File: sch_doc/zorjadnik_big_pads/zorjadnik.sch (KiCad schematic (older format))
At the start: 51 parts, among them J1 OUT1, J10 output GND, J11 power supply GND, J12 spare port, J2 OUT2, J3 Vsb, J4 GND, J5 display module, J6 firmware, J7 cooling fan, J9 power supply Vout, Q1 BCR512, Q2 BCR108, Q3 BCR108, U1 AP1117-33, U2 STM32F030F4Px

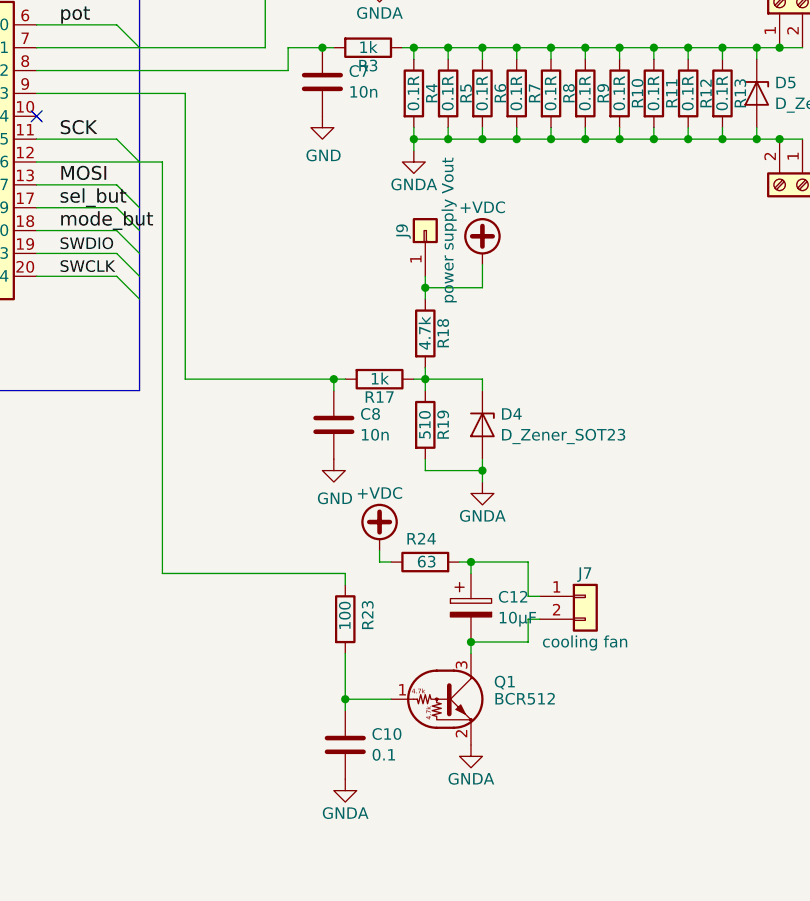
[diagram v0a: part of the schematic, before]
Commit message: что то подкрутил
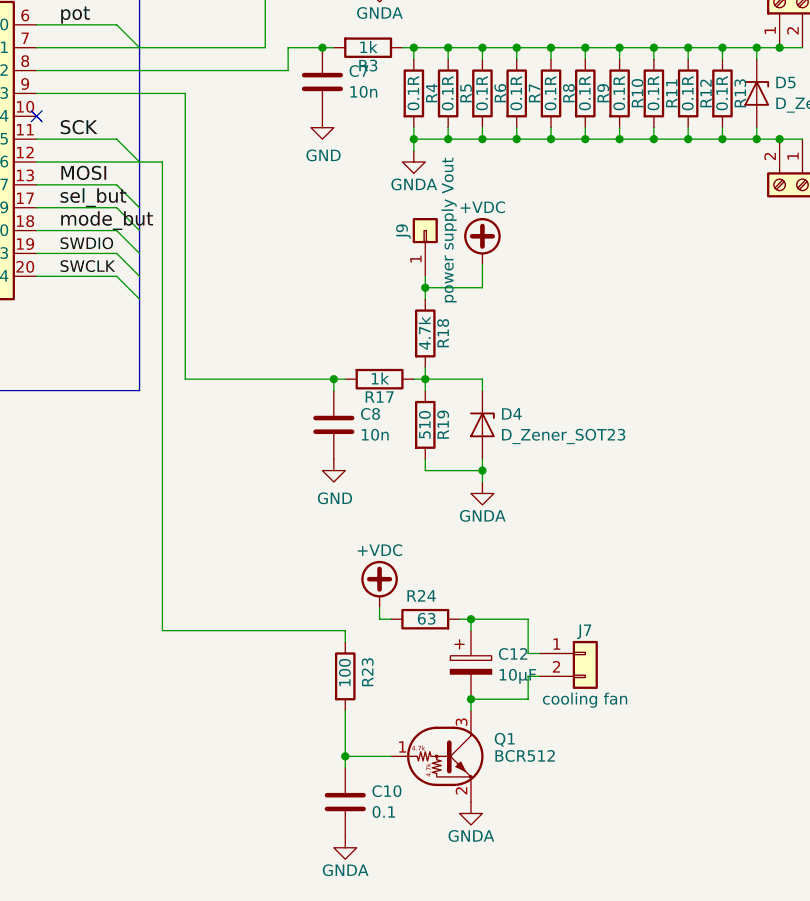
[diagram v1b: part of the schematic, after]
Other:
- moved on the sheet: C10, C12, J7, Q1, R23, R24
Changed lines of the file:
@@
 L led_digits:BCR512 Q1
 U 1 1 5D43E6DF
-P 6100 5900
-F 0 "Q1" H 6300 5975 50  0000 L CNN
-F 1 "BCR512" H 6300 5900 50  0000 L CNN
-F 2 "Package_TO_SOT_SMD:SOT-23" H 6100 5900 50  0001 L CNN
-F 3 "" H 6100 5900 50  0001 L CNN
-	1    6100 5900
+P 6100 6150
+F 0 "Q1" H 6300 6225 50  0000 L CNN
+F 1 "BCR512" H 6300 6150 50  0000 L CNN
+F 2 "Package_TO_SOT_SMD:SOT-23" H 6100 6150 50  0001 L CNN
+F 3 "" H 6100 6150 50  0001 L CNN
+	1    6100 6150
 	1    0    0    -1
 $EndComp
@@
 L zorjadnik-rescue:+VDC-power1 #PWR017
 U 1 1 5D43F586
-P 5800 5250
-F 0 "#PWR017" H 5800 5150 50  0001 C CNN
-F 1 "+VDC" H 5800 5500 50  0000 C CNN
-F 2 "" H 5800 5250 50  0001 C CNN
-F 3 "" H 5800 5250 50  0001 C CNN
-	1    5800 5250
-	1    0    0    -1
-$EndComp
-Wire Wire Line
-	5650 5900 5850 5900
+P 5800 5500
+F 0 "#PWR017" H 5800 5400 50  0001 C CNN
+F 1 "+VDC" H 5800 5750 50  0000 C CNN
+F 2 "" H 5800 5500 50  0001 C CNN
+F 3 "" H 5800 5500 50  0001 C CNN
+	1    5800 5500
+	1    0    0    -1
+$EndComp
+Wire Wire Line
+	5650 6150 5850 6150
 Entry Wire Line
 	4650 3650 4750 3750
@@
 L zorjadnik-rescue:GNDA-power1 #PWR0102
 U 1 1 5D598089
-P 6200 6100
-F 0 "#PWR0102" H 6200 5850 50  0001 C CNN
-F 1 "GNDA" H 6200 5950 50  0000 C CNN
-F 2 "" H 6200 6100 50  0001 C CNN
-F 3 "" H 6200 6100 50  0001 C CNN
-	1    6200 6100
+P 6200 6350
+F 0 "#PWR0102" H 6200 6100 50  0001 C CNN
+F 1 "GNDA" H 6200 6200 50  0000 C CNN
+F 2 "" H 6200 6350 50  0001 C CNN
+F 3 "" H 6200 6350 50  0001 C CNN
+	1    6200 6350
 	1    0    0    -1
 $EndComp
@@
 L zorjadnik-rescue:C-Device1 C10
 U 1 1 5D601FED
-P 5650 6100
-F 0 "C10" H 5765 6146 50  0000 L CNN
-F 1 "0.1" H 5765 6055 50  0000 L CNN
-F 2 "Capacitor_SMD:C_0603_1608Metric" H 5688 5950 50  0001 C CNN
-F 3 "~" H 5650 6100 50  0001 C CNN
-	1    5650 6100
+P 5650 6350
+F 0 "C10" H 5765 6396 50  0000 L CNN
+F 1 "0.1" H 5765 6305 50  0000 L CNN
+F 2 "Capacitor_SMD:C_0603_1608Metric" H 5688 6200 50  0001 C CNN
+F 3 "~" H 5650 6350 50  0001 C CNN
+	1    5650 6350
 	1    0    0    -1
 $EndComp
@@
 L zorjadnik-rescue:GNDA-power1 #PWR0106
 U 1 1 5D602460
-P 5650 6250
-F 0 "#PWR0106" H 5650 6000 50  0001 C CNN
-F 1 "GNDA" H 5650 6100 50  0000 C CNN
-F 2 "" H 5650 6250 50  0001 C CNN
-F 3 "" H 5650 6250 50  0001 C CNN
-	1    5650 6250
-	1    0    0    -1
-$EndComp
-Wire Wire Line
-	5650 5950 5650 5900
-Connection ~ 5650 5900
+P 5650 6500
+F 0 "#PWR0106" H 5650 6250 50  0001 C CNN
+F 1 "GNDA" H 5650 6350 50  0000 C CNN
+F 2 "" H 5650 6500 50  0001 C CNN
+F 3 "" H 5650 6500 50  0001 C CNN
+	1    5650 6500
+	1    0    0    -1
+$EndComp
+Wire Wire Line
+	5650 6200 5650 6150
+Connection ~ 5650 6150
 NoConn ~ 4300 3350
 Entry Wire Line
@@
 	5800 2750 5800 2700
 Wire Wire Line
-	4850 3550 4850 5350
-Wire Wire Line
-	4850 5350 5650 5350
+	4850 5600 5650 5600
 Wire Wire Line
 	5600 4500 4950 4500
@@
 	5300 2600 5450 2600
 Wire Wire Line
-	5650 5350 5650 5400
-Wire Wire Line
-	5650 5900 5650 5700
+	5650 5600 5650 5650
+Wire Wire Line
+	5650 6150 5650 5950
 $Comp
 L zorjadnik-rescue:R-Device1 R23
 U 1 1 5D4C7FD8
-P 5650 5550
-F 0 "R23" V 5750 5500 50  0000 L CNN
-F 1 "100" V 5650 5500 50  0000 L CNN
-F 2 "Resistor_SMD:R_0805_2012Metric" V 5580 5550 50  0001 C CNN
-F 3 "~" H 5650 5550 50  0001 C CNN
-	1    5650 5550
+P 5650 5800
+F 0 "R23" V 5750 5750 50  0000 L CNN
+F 1 "100" V 5650 5750 50  0000 L CNN
+F 2 "Resistor_SMD:R_0805_2012Metric" V 5580 5800 50  0001 C CNN
+F 3 "~" H 5650 5800 50  0001 C CNN
+	1    5650 5800
 	1    0    0    -1
 $EndComp
@@
 L zorjadnik-rescue:R-Device1 R24
 U 1 1 5DC2B8F0
-P 6000 5300
-F 0 "R24" V 6100 5250 50  0000 L CNN
-F 1 "63" V 6000 5250 50  0000 L CNN
-F 2 "Resistor_SMD:R_1206_3216Metric" V 5930 5300 50  0001 C CNN
-F 3 "~" H 6000 5300 50  0001 C CNN
-	1    6000 5300
+P 6000 5550
+F 0 "R24" V 6100 5500 50  0000 L CNN
+F 1 "63" V 6000 5500 50  0000 L CNN
+F 2 "Resistor_SMD:R_1206_3216Metric" V 5930 5550 50  0001 C CNN
+F 3 "~" H 6000 5550 50  0001 C CNN
+	1    6000 5550
 	0    -1   -1   0
 $EndComp
@@
 L zorjadnik-rescue:Conn_01x02-Connector_Generic1 J7
 U 1 1 5D4406AD
-P 6700 5450
-F 0 "J7" H 6700 5550 50  0000 C CNN
-F 1 "cooling fan" H 6700 5250 50  0000 C CNN
-F 2 "Connector_PinHeader_2.54mm:PinHeader_1x02_P2.54mm_Vertical" H 6700 5450 50  0001 C CNN
-F 3 "" H 6700 5450 50  0001 C CNN
-	1    6700 5450
+P 6700 5700
+F 0 "J7" H 6700 5800 50  0000 C CNN
+F 1 "cooling fan" H 6700 5500 50  0000 C CNN
+F 2 "Connector_PinHeader_2.54mm:PinHeader_1x02_P2.54mm_Vertical" H 6700 5700 50  0001 C CNN
+F 3 "" H 6700 5700 50  0001 C CNN
+	1    6700 5700
 	1    0    0    -1
 $EndComp
@@
 L zorjadnik-rescue:CP-Device1 C12
 U 1 1 5DF08F00
-P 6200 5500
-F 0 "C12" H 6318 5546 50  0000 L CNN
-F 1 "10µF" H 6318 5455 50  0000 L CNN
-F 2 "Capacitor_SMD:C_1206_3216Metric" H 6238 5350 50  0001 C CNN
-F 3 "~" H 6200 5500 50  0001 C CNN
-	1    6200 5500
-	1    0    0    -1
-$EndComp
-Wire Wire Line
-	6200 5700 6200 5650
-Wire Wire Line
-	6500 5550 6450 5550
-Wire Wire Line
-	6450 5550 6450 5650
-Wire Wire Line
-	6450 5650 6200 5650
-Connection ~ 6200 5650
-Wire Wire Line
-	6500 5450 6450 5450
-Wire Wire Line
-	6450 5450 6450 5300
-Wire Wire Line
-	6450 5300 6200 5300
-Wire Wire Line
-	6200 5350 6200 5300
-Connection ~ 6200 5300
-Wire Wire Line
-	6200 5300 6150 5300
-Wire Wire Line
-	5850 5300 5800 5300
-Wire Wire Line
-	5800 5300 5800 5250
+P 6200 5750
+F 0 "C12" H 6318 5796 50  0000 L CNN
+F 1 "10µF" H 6318 5705 50  0000 L CNN
+F 2 "Capacitor_SMD:C_1206_3216Metric" H 6238 5600 50  0001 C CNN
+F 3 "~" H 6200 5750 50  0001 C CNN
+	1    6200 5750
+	1    0    0    -1
+$EndComp
+Wire Wire Line
+	6200 5950 6200 5900
+Wire Wire Line
+	6500 5800 6450 5800
+Wire Wire Line
+	6450 5800 6450 5900
+Wire Wire Line
+	6450 5900 6200 5900
+Connection ~ 6200 5900
+Wire Wire Line
+	6500 5700 6450 5700
+Wire Wire Line
+	6450 5700 6450 5550
+Wire Wire Line
+	6450 5550 6200 5550
+Wire Wire Line
+	6200 5600 6200 5550
+Connection ~ 6200 5550
+Wire Wire Line
+	6200 5550 6150 5550
+Wire Wire Line
+	5850 5550 5800 5550
+Wire Wire Line
+	5800 5550 5800 5500
 Wire Wire Line
 	2750 3550 2750 3700
@@
 	2500 3550 2750 3550
 Wire Wire Line
+	4850 3550 4850 5600
+Wire Wire Line
 	4300 3550 4850 3550
